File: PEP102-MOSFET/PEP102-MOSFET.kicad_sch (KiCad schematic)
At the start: 14 parts, among them J1 Screw_Terminal_01x02, J2 Screw_Terminal_01x02, J3 Screw_Terminal_01x02, Q19 2N7002

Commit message: Done, kinda
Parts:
- J2: footprint PEP_library:TerminalBlock_Phoenix_MKDS-1,5-2-5.08_1x02_P5.08mm_Horizontal -> PEP_library:Screw terminal
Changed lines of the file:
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@@
 			)
 		)
-		(property "Footprint" "PEP_library:TerminalBlock_Phoenix_MKDS-1,5-2-5.08_1x02_P5.08mm_Horizontal"
+		(property "Footprint" "PEP_library:Screw terminal"
 			(at 160.02 39.37 0)
 			(effects

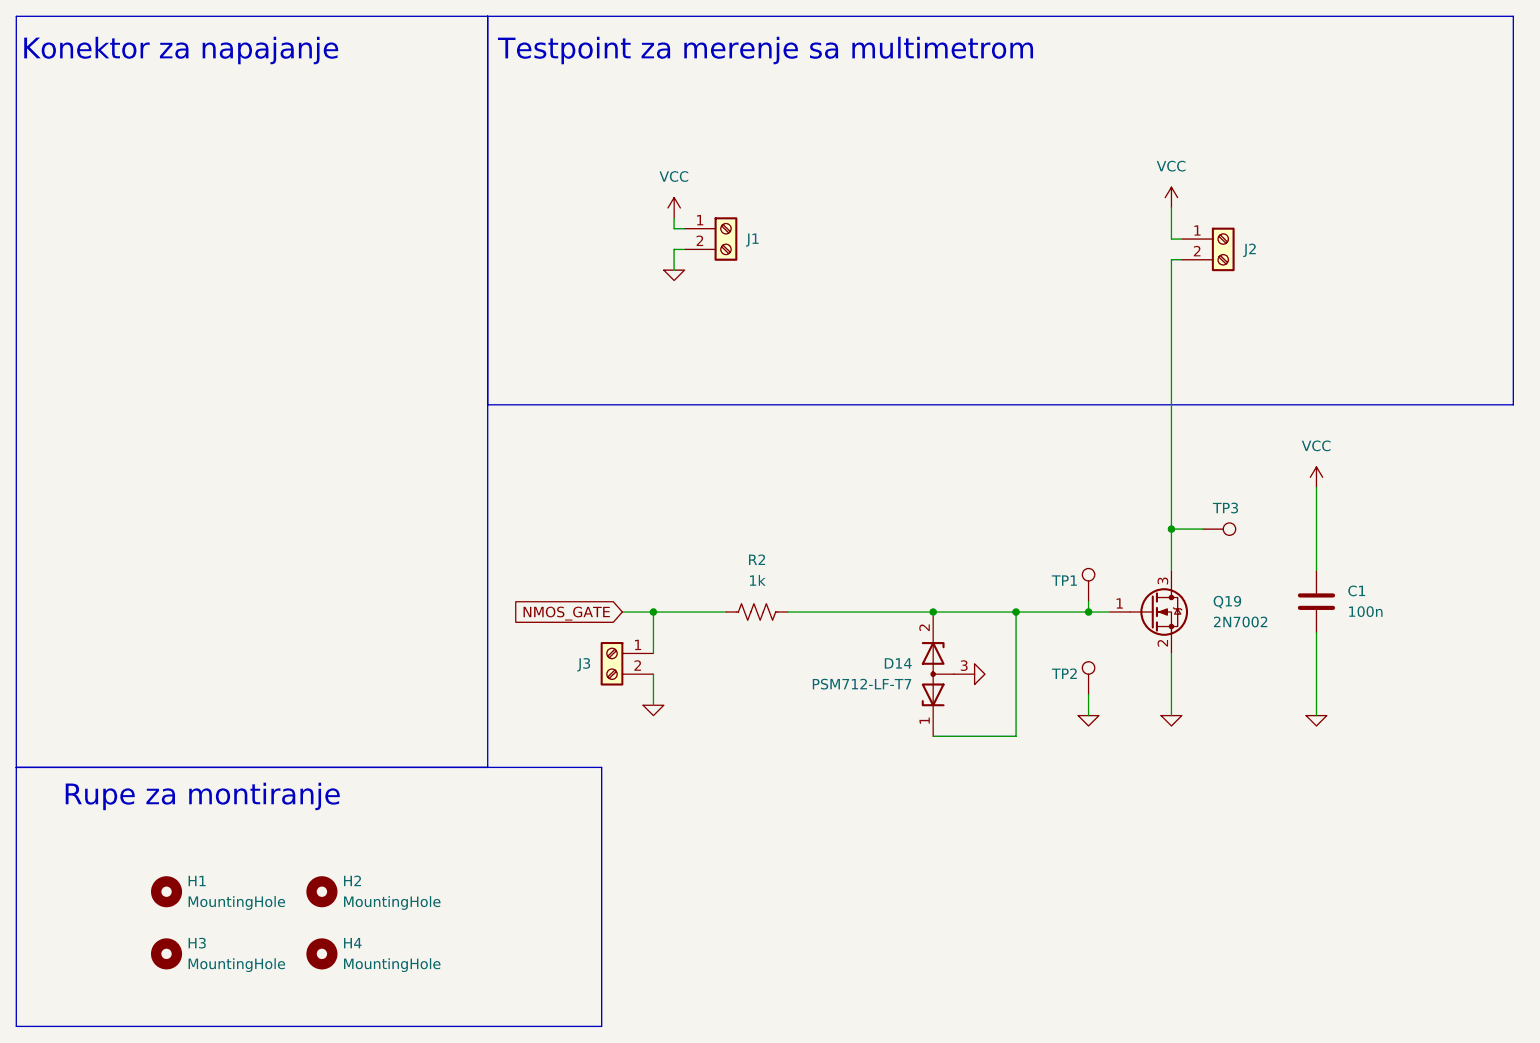
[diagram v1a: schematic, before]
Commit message: Done, kinda
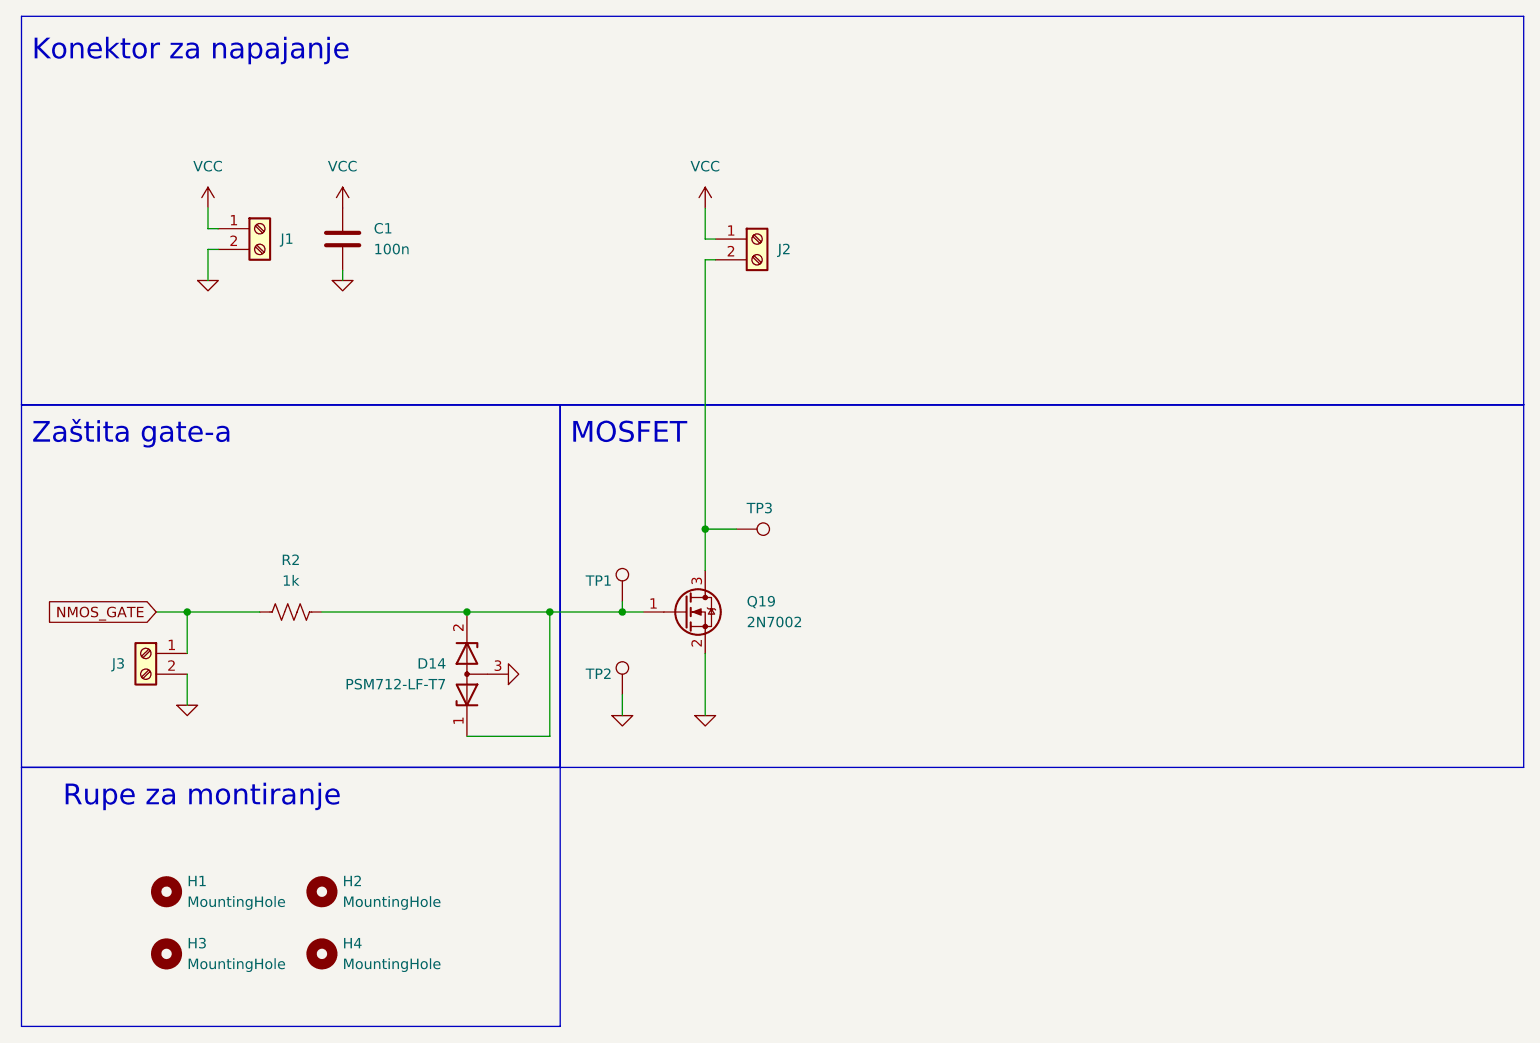
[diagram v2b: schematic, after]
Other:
- note added: "MOSFET"
- note added: "Zaštita gate-a"
- note removed: "Testpoint za merenje sa multimetrom"
- moved on the sheet: C1, D14, J1, J2, J3, Q19, R2, TP1, TP2, TP3
